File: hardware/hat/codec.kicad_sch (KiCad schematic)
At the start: 62 parts, among them J3 LineIn, J4 LineOut, J5 Headphone, U4 MAX98089ETN_T, Y1 12.288MHz

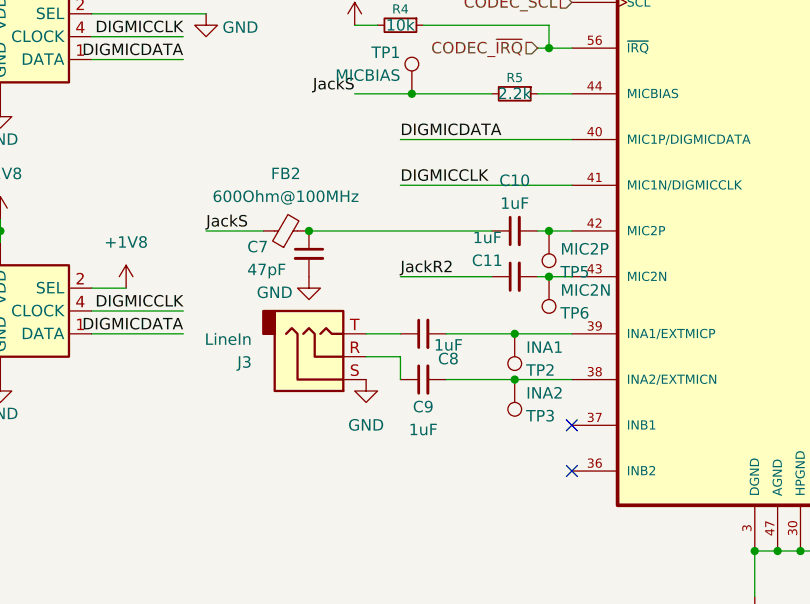
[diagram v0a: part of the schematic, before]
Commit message: hw: placement
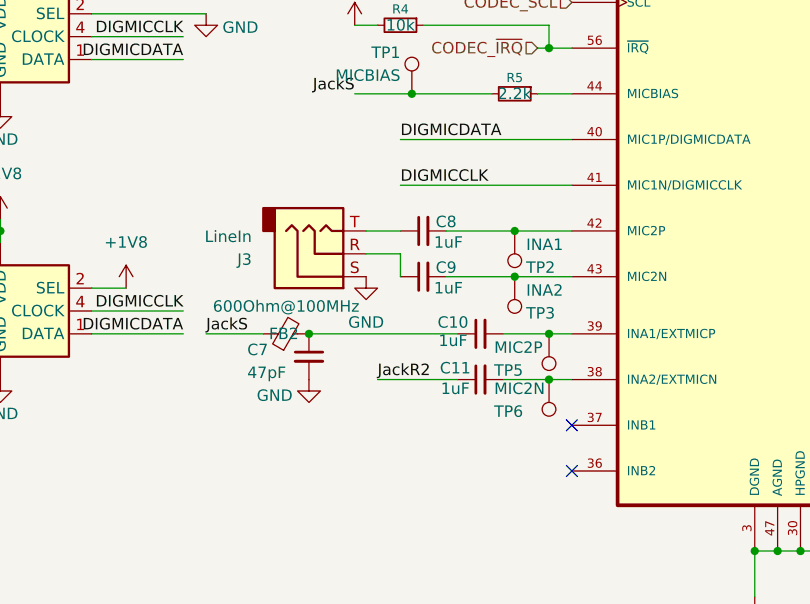
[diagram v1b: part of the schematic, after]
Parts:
- J3, J4: footprint Connector_Audio:Jack_3.5mm_PJ311_Horizontal -> Connector_Audio:Jack_3.5mm_CUI_SJ-3523-SMT_Horizontal
- J5: footprint Connector_Audio:Jack_3.5mm_PJ320D_Horizontal -> footprints:CUI_SJ-43514-SMT-TR
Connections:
- net at C10.2, TP5.1: now also U4.39 (INA1/EXTMICP); no longer U4.42 (MIC2P)
- net at C9.2, TP3.1: now also U4.43 (MIC2N); no longer U4.38 (INA2/EXTMICN)
- net at C8.2, TP2.1: now also U4.42 (MIC2P); no longer U4.39 (INA1/EXTMICP)
- net at C11.2, TP6.1: now also U4.38 (INA2/EXTMICN); no longer U4.43 (MIC2N)
